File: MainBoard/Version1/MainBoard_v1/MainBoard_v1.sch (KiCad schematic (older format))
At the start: 165 parts, among them J1 ILG, J10 SH, J11 SH, J12 SH, J13 FFC, J14 SH, J2 SH, J3 SH, J4 PA, J5 Micro_SD_Card_Det_Hirose_DM3AT, J6 SH, J7 ENC, J8 ENC, J9 PA, Q1 AON7400B, Q10 IRLML6344, Q2 AON7400B, Q3 AON7400B, Q4 AON7400B, Q5 AON7400B, Q6 AON7400B, Q7 2N7002K, Q8 AON7400B, Q9 AON7400B, SW1 SKRPACE010, SW2 SSSS213202, SW3 FR01SC16P-S, SW4 SKRHAAE010, U1 SI7469DP-T1-GE3, U10 DRV8701E, U11 MMC5983MA, U2 LT1963A-TSSOP, U3 TPS62143, U4 ECS-2520S33, U5 INA260, U6 DRV8701E, U7 ICM20648, U8 STM32F469VG, U9 INA260

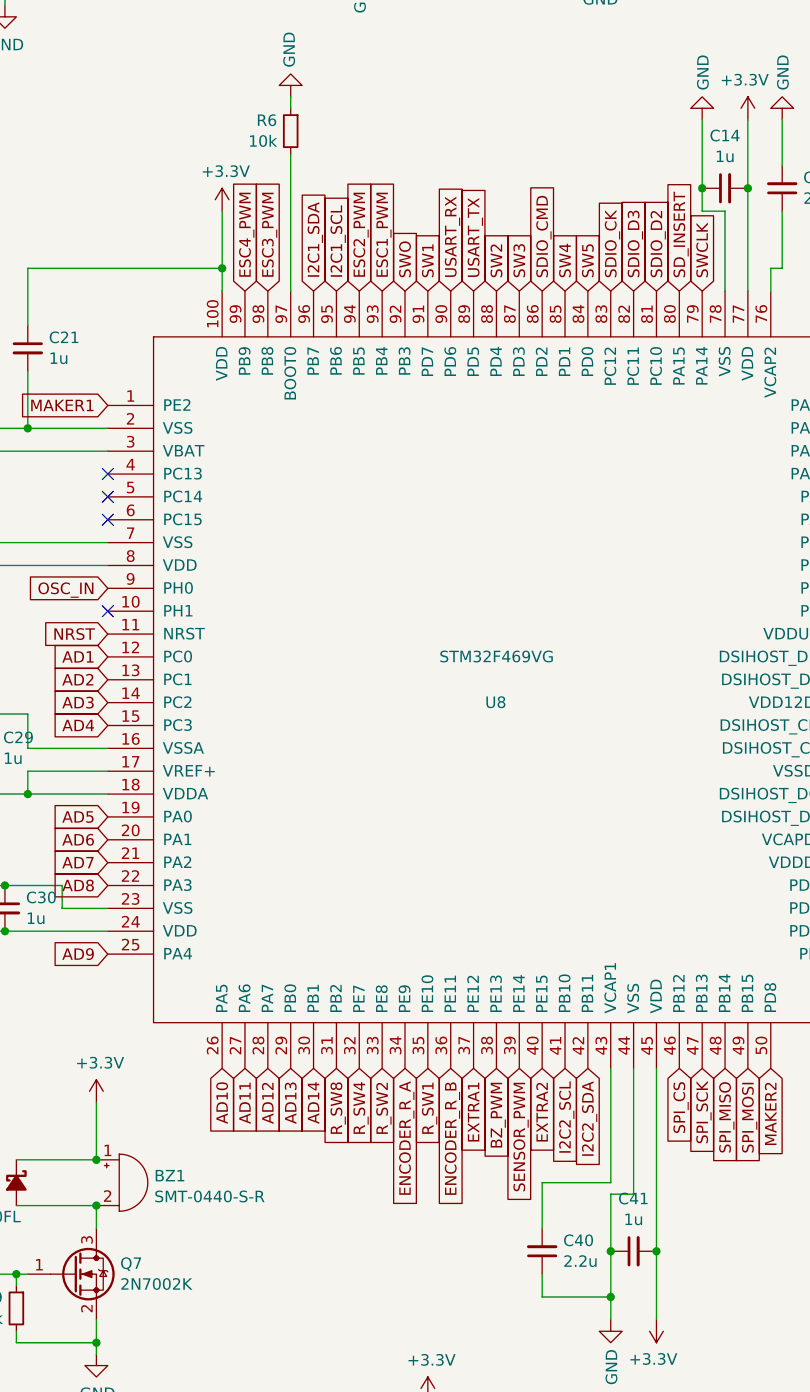
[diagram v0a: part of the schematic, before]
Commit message: commit
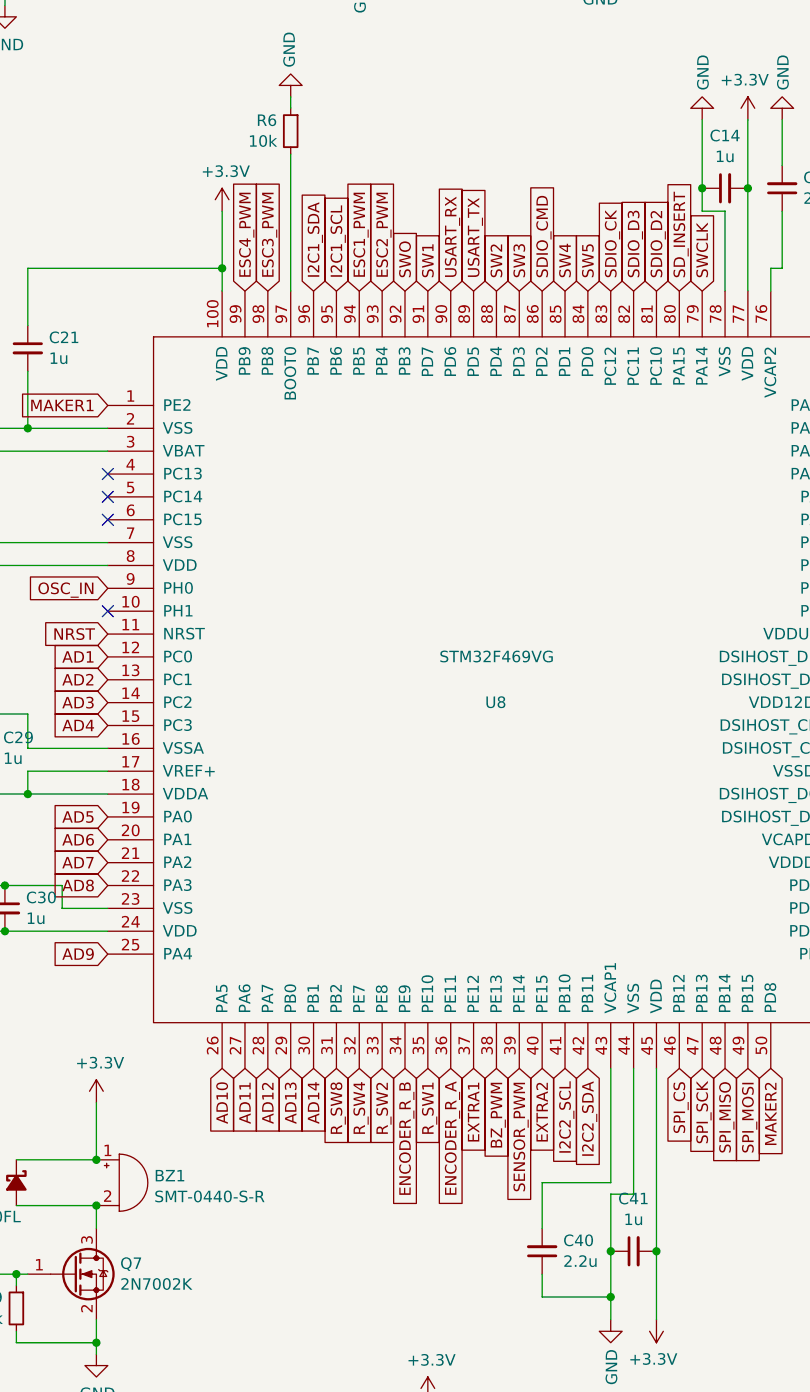
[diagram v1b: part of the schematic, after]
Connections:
- net ENCODER_R_A: now also U8.36 (PE11); no longer U8.34 (PE9)
- net ENCODER_R_B: now also U8.34 (PE9); no longer U8.36 (PE11)
- net ESC1_PWM: now also U8.94 (PB5); no longer U8.93 (PB4)
- net ESC2_PWM: now also U8.93 (PB4); no longer U8.94 (PB5)
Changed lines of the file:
@@
 Text GLabel 5450 4300 2    50   Input ~ 0
 LED_B
+Text GLabel 3550 6900 3    50   Input ~ 0
+ENCODER_R_A
 Text GLabel 3350 6900 3    50   Input ~ 0
-ENCODER_R_A
-Text GLabel 3550 6900 3    50   Input ~ 0
 ENCODER_R_B
 Text GLabel 4150 6900 3    50   Input ~ 0
@@
 Text GLabel 3450 3500 1    50   Input ~ 0
 SW1
+Text GLabel 3150 3500 1    50   Input ~ 0
+ESC1_PWM
 Text GLabel 3250 3500 1    50   Input ~ 0
-ESC1_PWM
-Text GLabel 3150 3500 1    50   Input ~ 0
 ESC2_PWM
 Text GLabel 3050 3500 1    50   Input ~ 0
